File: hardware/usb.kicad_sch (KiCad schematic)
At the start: 5 parts

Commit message: Fix BOM entries, should be good to go
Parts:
- C25: LCSC Part (none) -> C1525
- R19, R20: LCSC Part (none) -> C25905
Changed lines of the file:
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@@
+			)
+		)
+		(property "LCSC Part" "C1525"
+			(at 171.45 74.93 0)
+			(effects
+				(font
+					(size 1.27 1.27)
+				)
+				(hide yes)
 			)
 		)
@@
 			)
 		)
+		(property "LCSC Part" "C25905"
+			(at 127 118.11 0)
+			(effects
+				(font
+					(size 1.27 1.27)
+				)
+				(hide yes)
+			)
+		)
 		(pin "1"
 		)
@@
 			(at 139.7 118.11 0)
 			(effects
+				(font
+					(size 1.27 1.27)
+				)
+				(hide yes)
+			)
+		)
+		(property "LCSC Part" "C25905"
+			(at 139.7 118.11 0)
+			(effects

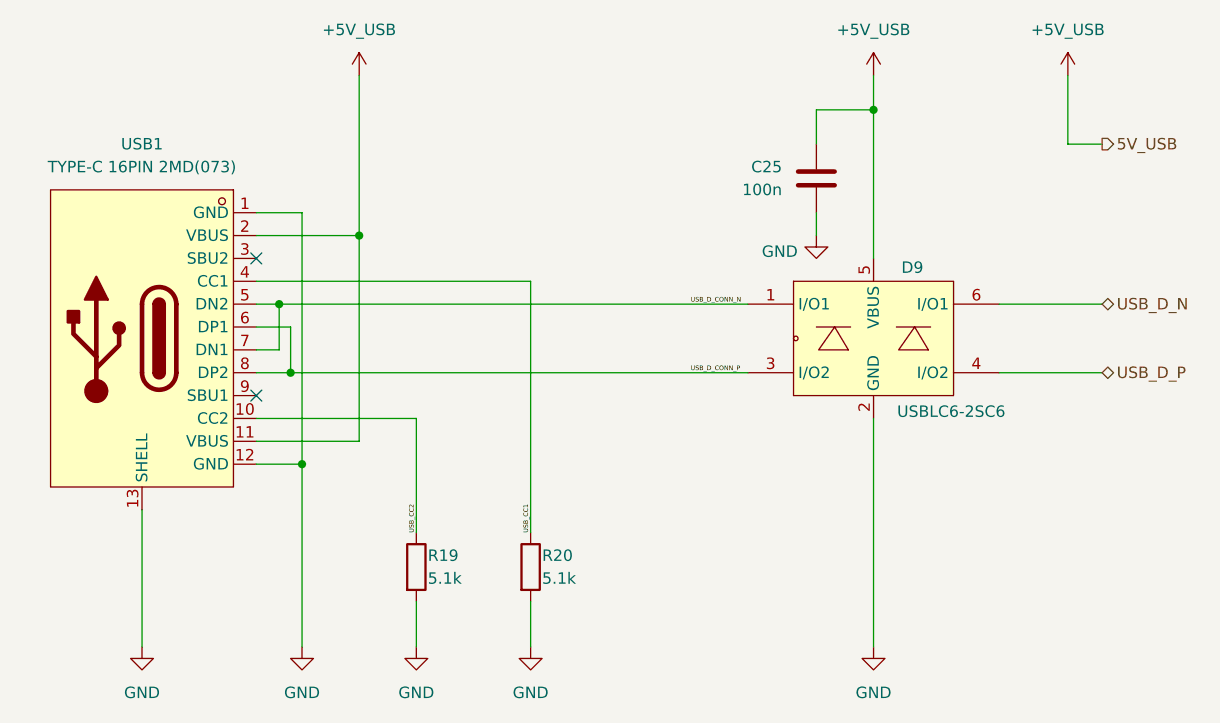
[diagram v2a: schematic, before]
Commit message: First of listed hardware changes, need verification
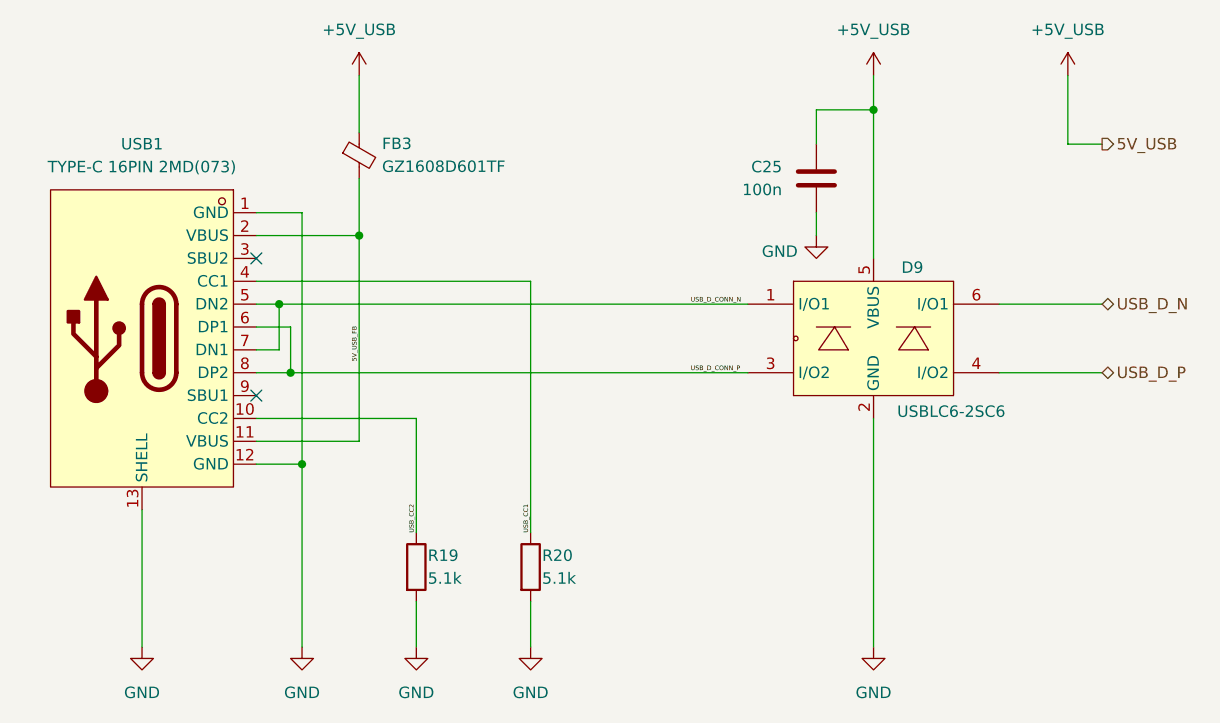
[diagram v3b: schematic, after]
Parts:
- added FB3: GZ1608D601TF, Resistor_SMD:R_0603_1608Metric, symbol Device:FerriteBead_Small
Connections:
- net +5V_USB: now also FB3.1; no longer USB1.11 (VBUS), USB1.2 (VBUS)
- new net 5V_USB_FB: FB3.2, USB1.11 (VBUS), USB1.2 (VBUS)
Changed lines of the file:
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@@
+	(wire
+		(pts
+			(xy 120.65 81.28) (xy 120.65 104.14)
+		)
+		(stroke
+			(width 0)
+			(type default)
+		)
+	)
 	(wire
 		(pts
@@
 	(wire
 		(pts
-			(xy 120.65 63.5) (xy 120.65 81.28)
+			(xy 120.65 63.5) (xy 120.65 69.85)
 		)
 		(stroke
@@
 	(wire
 		(pts
-			(xy 120.65 104.14) (xy 120.65 81.28)
-		)
-		(stroke
-			(width 0)
-			(type default)
-		)
-	)
-	(wire
-		(pts
 			(xy 109.22 88.9) (xy 111.76 88.9)
 		)
@@
 	(wire
 		(pts
+			(xy 120.65 74.93) (xy 120.65 81.28)
+		)
+		(stroke
+			(width 0)
+			(type default)
+		)
+	)
+	(wire
+		(pts
 			(xy 109.22 104.14) (xy 120.65 104.14)
 		)
@@
 			(width 0)
 			(type default)
+		)
+	)
+	(label "5V_USB_FB"
+		(at 120.65 95.25 90)
+		(effects
+			(font
+				(size 0.508 0.508)
+				(color 132 132 132 1)
+			)
+			(justify left bottom)
 		)
 	)
@@
 					(unit 1)
 				)
+			)
+		)
+	)
+	(symbol
+		(lib_id "Device:FerriteBead_Small")
+		(at 120.65 72.39 0)
+		(unit 1)
+		(exclude_from_sim no)
+		(in_bom yes)
+		(on_board yes)
+		(dnp no)
+		(fields_autoplaced yes)
+		(property "Reference" "FB3"
+			(at 123.19 71.0818 0)
+			(effects
+				(font
+					(size 1.27 1.27)
+				)
+				(justify left)
+			)
+		)
+		(property "Value" "GZ1608D601TF"
+			(at 123.19 73.6218 0)
+			(effects
+				(font
+					(size 1.27 1.27)
+				)
+				(justify left)
+			)
+		)
+		(property "Footprint" "Resistor_SMD:R_0603_1608Metric"
+			(at 118.872 72.39 90)
+			(effects
+				(font
+					(size 1.27 1.27)
+				)
+				(hide yes)
+			)
+		)
+		(property "Datasheet" "~"
+			(at 120.65 72.39 0)
+			(effects
+				(font
+					(size 1.27 1.27)
+				)
+				(hide yes)
+			)
+		)
+		(property "Description" "GZ1608D601TF"
+			(at 120.65 72.39 0)
+			(effects
+				(font
+					(size 1.27 1.27)
+				)
+				(hide yes)
+			)
+		)
+		(property "LCSC Part" "C1002"
+			(at 120.65 72.39 90)
+			(effects
+				(font
+					(size 1.27 1.27)
+				)
+				(hide yes)
+			)
+		)
+		(pin "2"
+		)
+		(pin "1"
+		)
+		(instances
+			(project "uPTP"
+				(path "/c29659fd-9e8d-4714-a690-4e74e6e849c2/a01e8bf2-a35e-4434-a60c-3e16f0eed29e"
+					(reference "FB3")
+					(unit 1)
+				)
